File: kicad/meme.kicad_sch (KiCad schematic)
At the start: 12 parts, among them U3 28C256, U4 74HC245D, U6 74HC245D, U7 74HC245D, U8 HM628128D_DIP32_SOP32, U9 CY62256-70PC

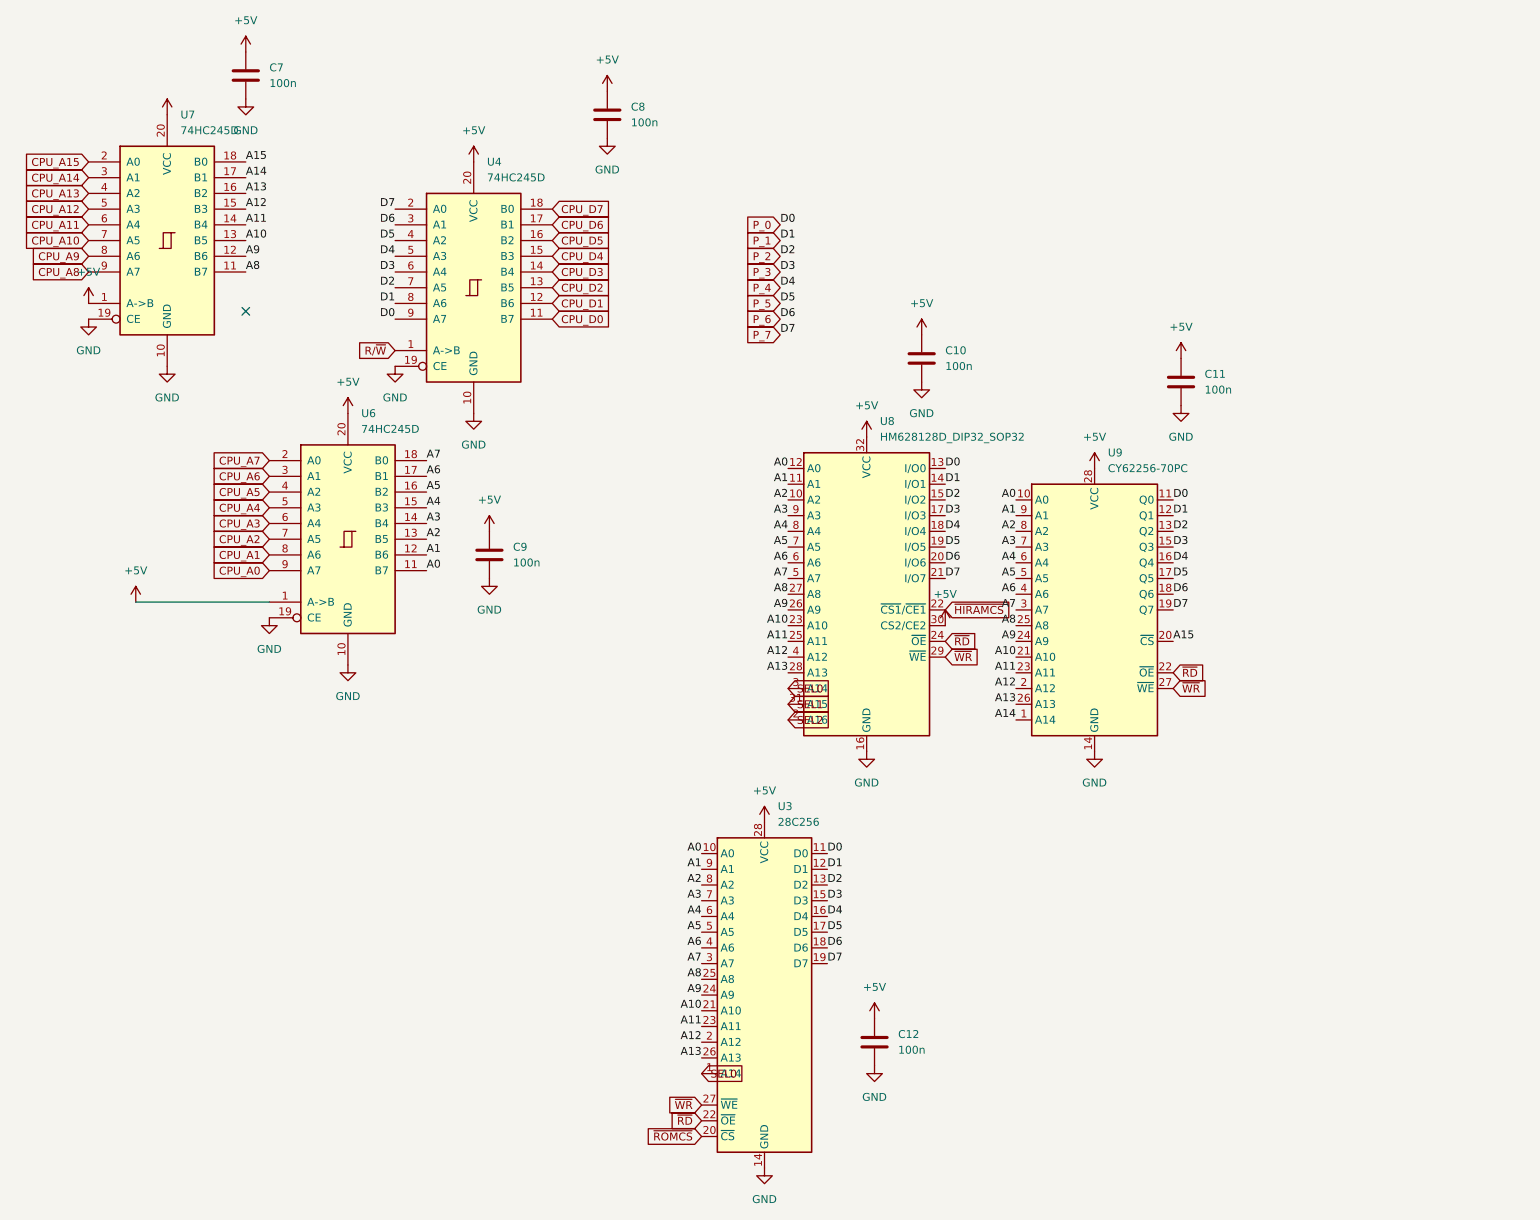
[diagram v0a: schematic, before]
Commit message: add third menu
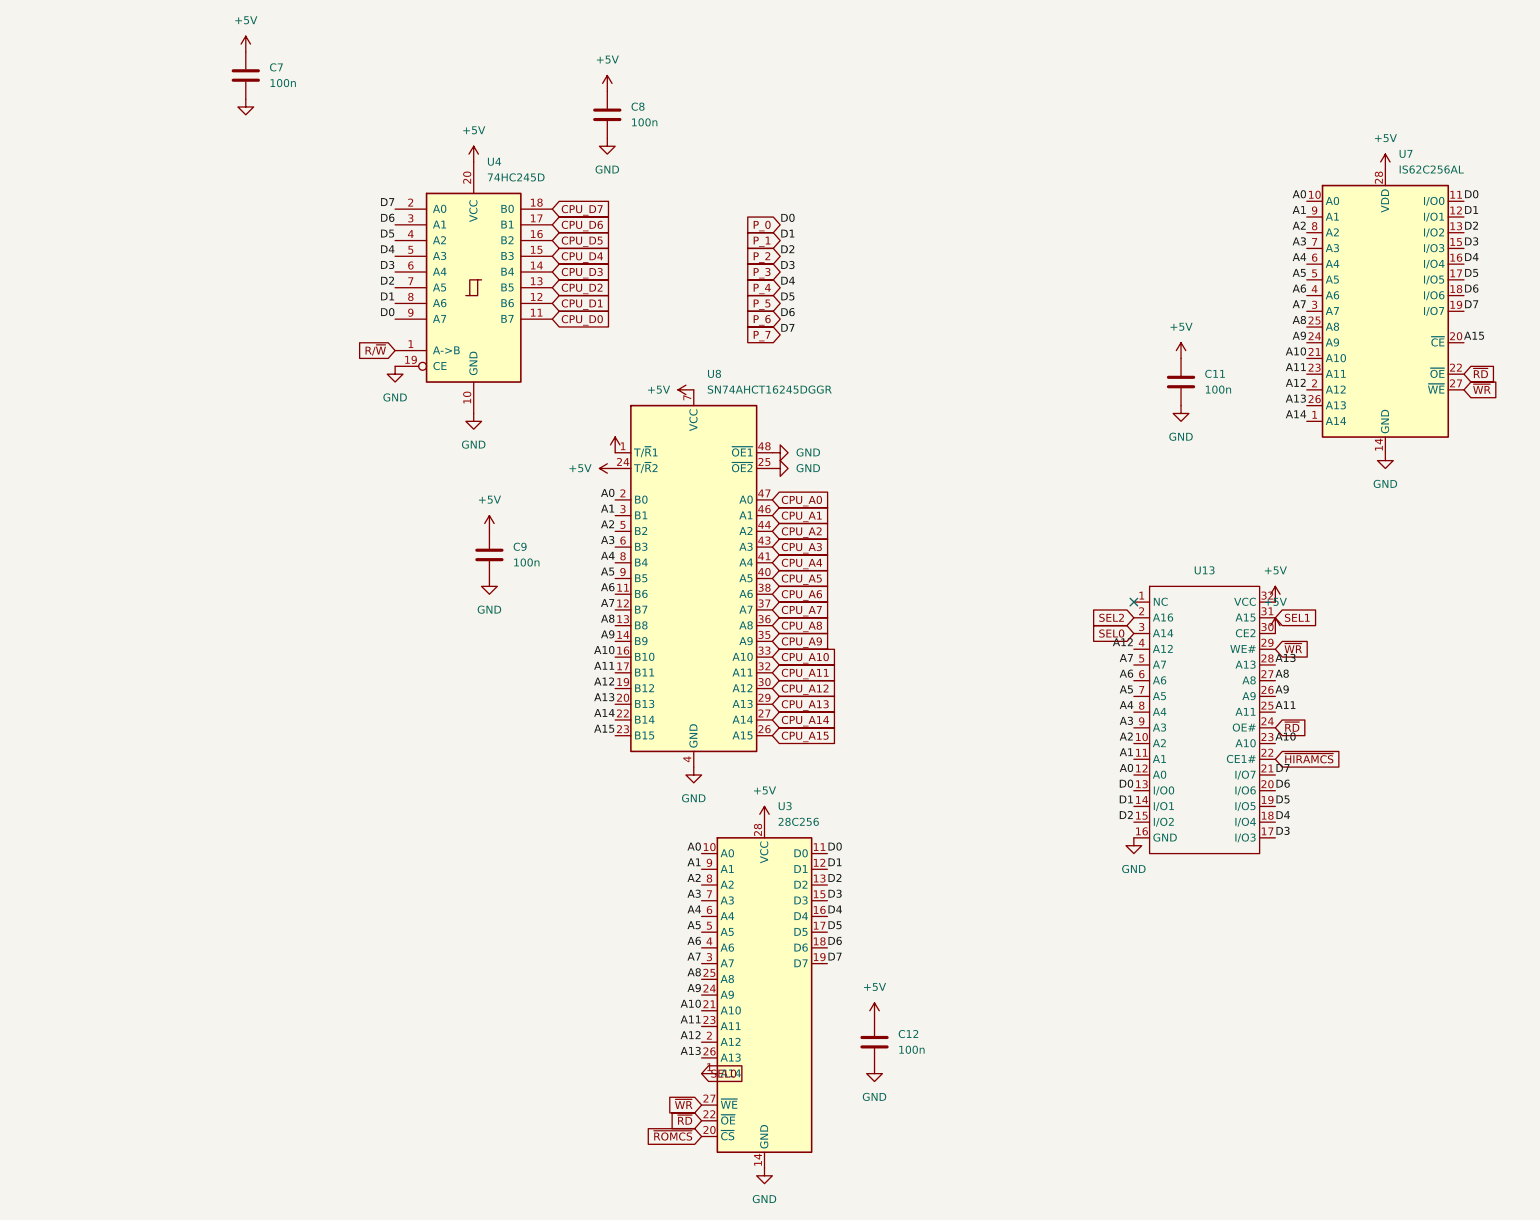
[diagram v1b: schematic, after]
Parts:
- removed C10: 100n, Capacitor_SMD:C_0603_1608Metric, symbol Device:C
- removed U6, U7: 74HC245D, Package_SO:SOIC-20W_7.5x12.8mm_P1.27mm, symbol 74xx:74HC245
- removed U8: HM628128D_DIP32_SOP32, Package_DIP:DIP-32_W15.24mm_Socket, symbol Memory_RAM:HM628128D_DIP32_SOP32
- removed U9: CY62256-70PC, Package_DIP:DIP-28_W15.24mm_Socket, symbol Memory_RAM:CY62256-70PC
- added U13: (no value), Package_SO:SOJ-32_7.62x20.955mm_P1.27mm, symbol EasyEDA_Lib:CY7C1009D-10VXIT
- added U7: IS62C256AL, Package_SO:SOP-28_8.4x18.16mm_P1.27mm, symbol Memory_RAM:IS62C256AL
- added U8: SN74AHCT16245DGGR, Package_SO:TSSOP-48_6.1x12.5mm_P0.5mm, symbol 74xx:MC74LCX16245DT
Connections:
- net +5V: now also U13.30 (CE2), U13.32 (VCC), U7.28 (VDD), U8.1 (T/~{R}1), U8.18 (VCC), U8.24 (T/~{R}2), U8.31 (VCC), U8.42 (VCC), U8.7 (VCC)
- net A0: now also U13.12 (A0), U7.10 (A0), U8.2 (B0)
- net A1: now also U13.11 (A1), U7.9 (A1), U8.3 (B1)
- net A10: now also U13.23 (A10), U7.21 (A10), U8.16 (B10)
- net A11: now also U13.25 (A11), U7.23 (A11), U8.17 (B11)
- net A12: now also U13.4 (A12), U7.2 (A12), U8.19 (B12)
- net A13: now also U13.28 (A13), U7.26 (A13), U8.20 (B13)
- net A14: now also U7.1 (A14), U8.22 (B14)
- net A15: now also U7.20 (~{CE}), U8.23 (B15)
- net A2: now also U13.10 (A2), U7.8 (A2), U8.5 (B2)
- net A3: now also U13.9 (A3), U7.7 (A3), U8.6 (B3)
- net A4: now also U13.8 (A4), U7.6 (A4), U8.8 (B4)
- net A5: now also U13.7 (A5), U7.5 (A5), U8.9 (B5)
- net A6: now also U13.6 (A6), U7.4 (A6), U8.11 (B6)
- net A7: now also U13.5 (A7), U7.3 (A7), U8.12 (B7)
- net A8: now also U13.27 (A8), U7.25 (A8), U8.13 (B8)
- net A9: now also U13.26 (A9), U7.24 (A9), U8.14 (B9)
- net CPU_A0: now also U8.47 (A0)
- net CPU_A1: now also U8.46 (A1)
- net CPU_A10: now also U8.33 (A10)
- net CPU_A11: now also U8.32 (A11)
- net CPU_A12: now also U8.30 (A12)
- net CPU_A13: now also U8.29 (A13)
- net CPU_A14: now also U8.27 (A14)
- net CPU_A15: now also U8.26 (A15)
- net CPU_A2: now also U8.44 (A2)
- net CPU_A3: now also U8.43 (A3)
- net CPU_A4: now also U8.41 (A4)
- net CPU_A5: now also U8.40 (A5)
- net CPU_A6: now also U8.38 (A6)
- net CPU_A7: now also U8.37 (A7)
- net CPU_A8: now also U8.36 (A8)
- net CPU_A9: now also U8.35 (A9)
- net GND: now also U13.16 (GND), U7.14 (GND), U8.10 (GND), U8.15 (GND), U8.21 (GND), U8.25 (~{OE2}), U8.28 (GND), U8.34 (GND), U8.39 (GND), U8.4 (GND), U8.45 (GND), U8.48 (~{OE1})
- net P_0: now also U13.13 (I/O0), U7.11 (I/O0)
- net P_1: now also U13.14 (I/O1), U7.12 (I/O1)
- net P_2: now also U13.15 (I/O2), U7.13 (I/O2)
- net P_3: now also U13.17 (I/O3), U7.15 (I/O3)
- net P_4: now also U13.18 (I/O4), U7.16 (I/O4)
- net P_5: now also U13.19 (I/O5), U7.17 (I/O5)
- net P_6: now also U13.20 (I/O6), U7.18 (I/O6)
- net P_7: now also U13.21 (I/O7), U7.19 (I/O7)
- net SEL0: now also U13.3 (A14)
- net SEL1: now also U13.31 (A15)
- net SEL2: now also U13.2 (A16)
- net ~{HIRAMCS}: now also U13.22 (CE1#)
- net ~{RD}: now also U13.24 (OE#), U7.22 (~{OE})
- net ~{WR}: now also U13.29 (WE#), U7.27 (~{WE})
